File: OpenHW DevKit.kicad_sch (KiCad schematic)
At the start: 69 parts, among them J10 Conn_01x20, J4 Conn_01x02_Male, J7 Conn_01x20, J8 Conn_01x20, J9 Conn_01x20, Q1 MMBT3904, Q2 MMBT3904, SW1 SW_Push, SW2 SW_Push, U14 CORE-V-MCU, U3 W25Q32JWZP, U4 FXMA2102UMX, U6 NTB0104BQ,115, U7 NTB0104BQ,115, U8 NTB0104BQ,115, U9 NTB0104BQ,115, X1 ECS-2520MVLC-100-CN

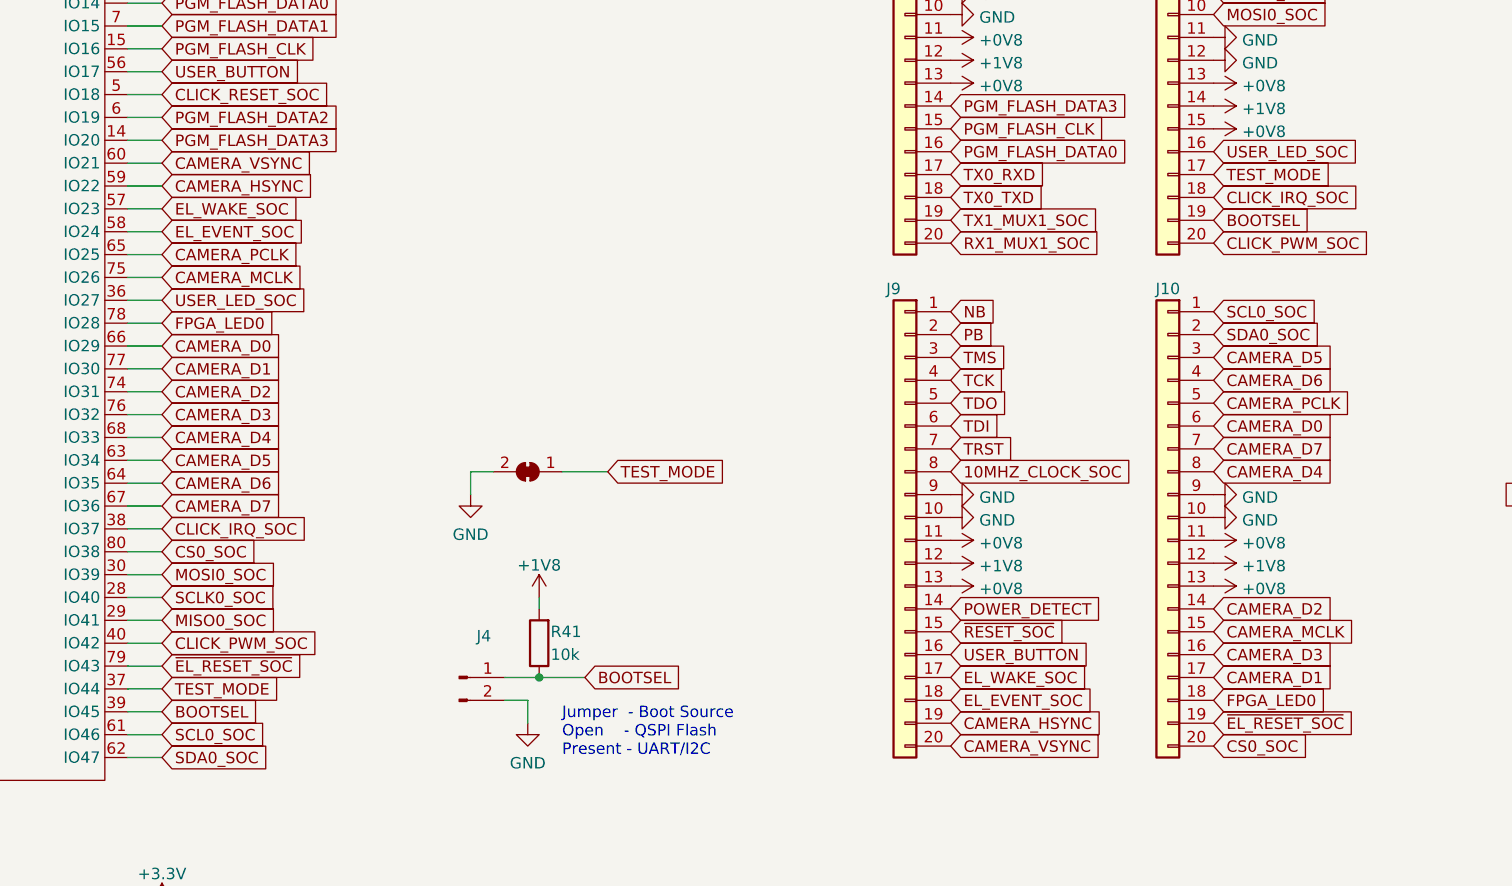
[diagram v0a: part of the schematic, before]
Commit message: swapped bootsel & test_mode pins
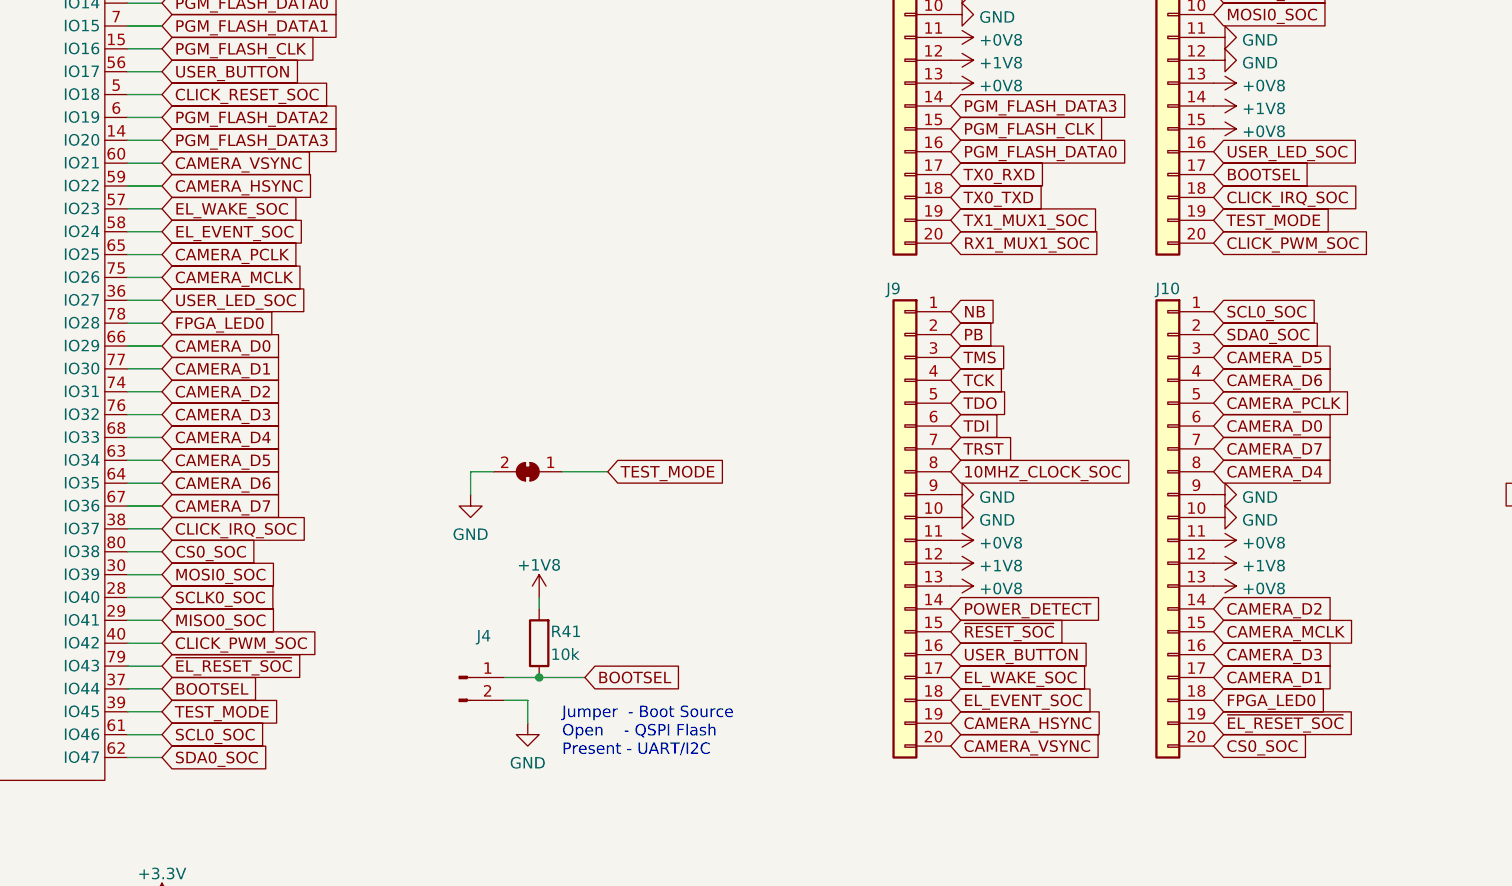
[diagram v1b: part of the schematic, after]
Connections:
- net BOOTSEL: now also J8.17 (Pin_17), U14.37 (IO44); no longer J8.19 (Pin_19), U14.39 (IO45)
- net TEST_MODE: now also J8.19 (Pin_19), U14.39 (IO45); no longer J8.17 (Pin_17), U14.37 (IO44)

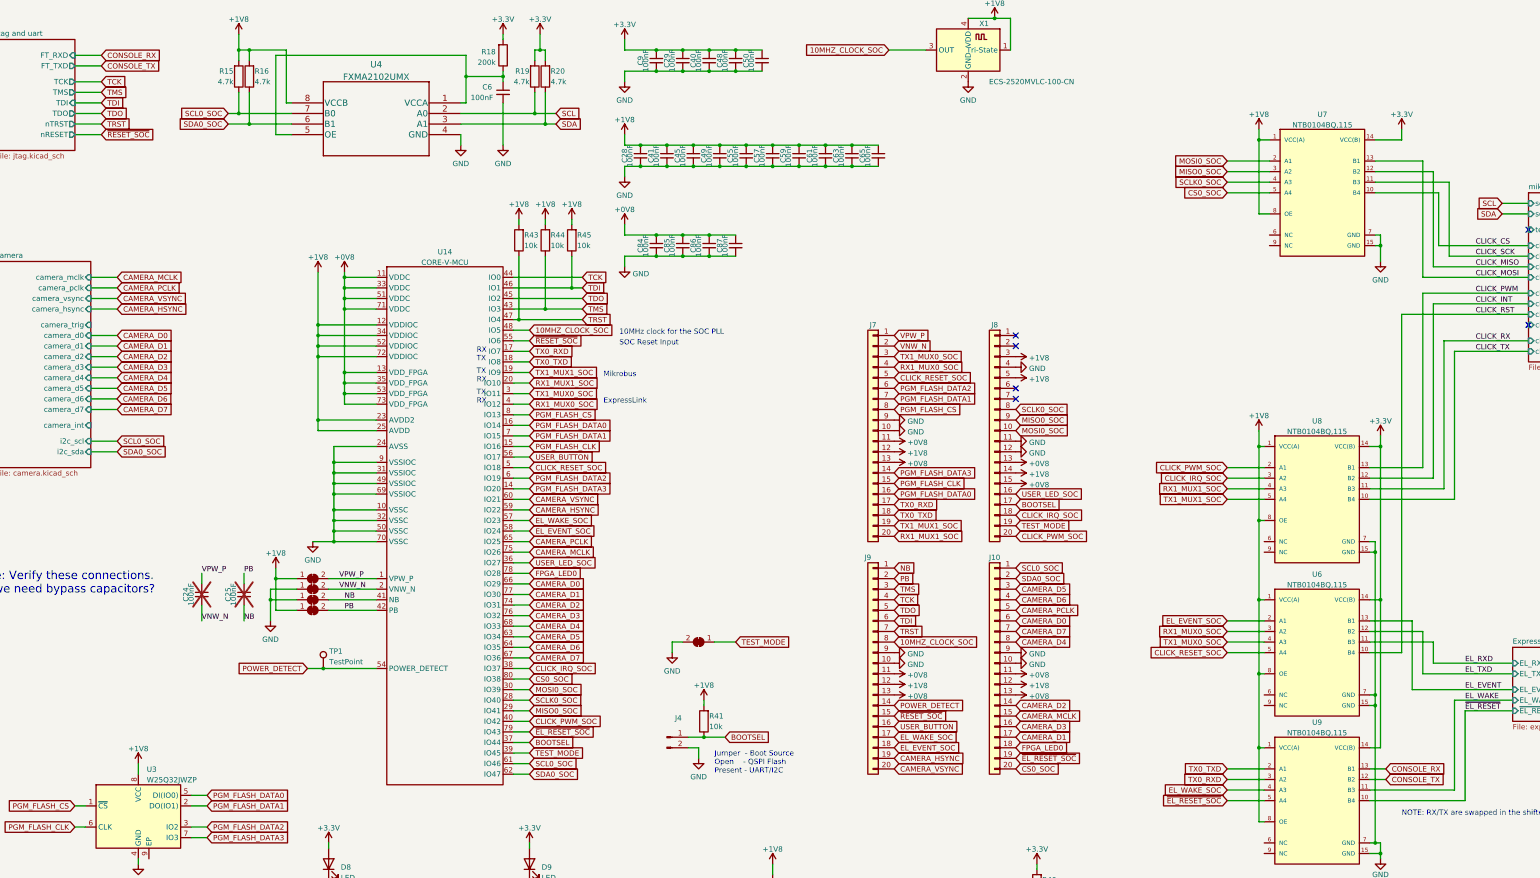
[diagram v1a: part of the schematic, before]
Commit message: updated footprints, added the barrel power connector and test points
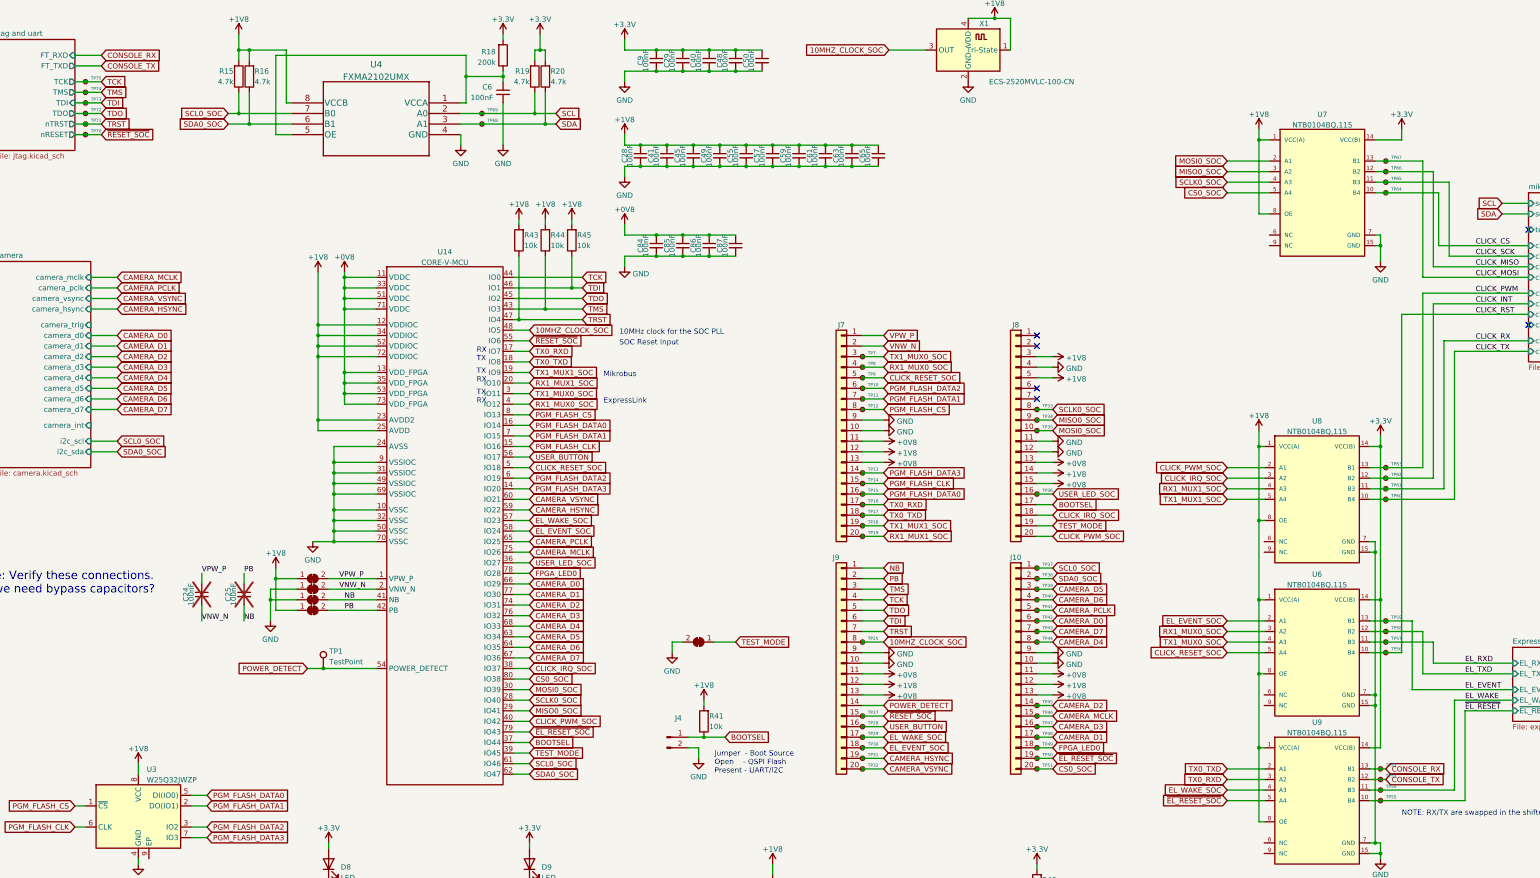
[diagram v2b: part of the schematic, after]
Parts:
- added TP10, TP11, TP12, TP13, TP14, TP15, TP16, TP17, TP18, TP19, TP25, TP27, TP28, TP29, TP30, TP31, TP32, TP33, TP34, TP35, TP36, TP37, TP38, TP39, TP40, TP41, TP42, TP43, TP44, TP45, TP46, TP47, TP48, TP49, TP50, TP51, TP52, TP53, TP54, TP55, TP56, TP57, TP58, TP59, TP60, TP61, TP62, TP63, TP64, TP65, TP66, TP67, TP68, TP69, TP7, TP70, TP71, TP72, TP73, TP74, TP75, TP8, TP9: TestPoint_Small, TestPoint:TestPoint_Pad_D1.0mm, symbol Connector:TestPoint_Small
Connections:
- net 10MHZ_CLOCK_SOC: now also TP25.1
- net CAMERA_D0: now also TP42.1
- net CAMERA_D1: now also TP48.1
- net CAMERA_D2: now also TP45.1
- net CAMERA_D3: now also TP47.1
- net CAMERA_D4: now also TP44.1
- net CAMERA_D5: now also TP39.1
- net CAMERA_D6: now also TP40.1
- net CAMERA_D7: now also TP43.1
- net CAMERA_HSYNC: now also TP31.1
- net CAMERA_MCLK: now also TP46.1
- net CAMERA_PCLK: now also TP41.1
- net CAMERA_VSYNC: now also TP32.1
- net CLICK_CS: now also TP64.1
- net CLICK_INT: now also TP62.1
- net CLICK_MISO: now also TP66.1
- net CLICK_MOSI: now also TP67.1
- net CLICK_PWM: now also TP63.1
- net CLICK_RESET_SOC: now also TP9.1
- net CLICK_RST: now also TP56.1
- net CLICK_RX: now also TP61.1
- net CLICK_SCK: now also TP65.1
- net CLICK_TX: now also TP60.1
- net CONSOLE_RX: now also TP52.1
- net CONSOLE_TX: now also TP53.1
- net CS0_SOC: now also TP51.1
- net EL_EVENT: now also TP59.1
- net EL_EVENT_SOC: now also TP30.1
- net EL_RXD: now also TP57.1
- net EL_TXD: now also TP58.1
- net EL_WAKE: now also TP54.1
- net EL_WAKE_SOC: now also TP29.1
- net FPGA_LED0: now also TP49.1
- net MISO0_SOC: now also TP34.1
- net MOSI0_SOC: now also TP35.1
- net PGM_FLASH_CLK: now also TP14.1
- net PGM_FLASH_CS: now also TP12.1
- net PGM_FLASH_DATA0: now also TP15.1
- net PGM_FLASH_DATA1: now also TP11.1
- net PGM_FLASH_DATA2: now also TP10.1
- net PGM_FLASH_DATA3: now also TP13.1
- net RX1_MUX0_SOC: now also TP8.1
- net RX1_MUX1_SOC: now also TP19.1
- net SCL: now also TP69.1
- net SCL0_SOC: now also TP37.1
- net SCLK0_SOC: now also TP33.1
- net SDA: now also TP68.1
- net SDA0_SOC: now also TP38.1
- net TCK: now also TP75.1
- net TDI: now also TP73.1
- net TDO: now also TP72.1
- net TMS: now also TP74.1
- net TRST: now also TP71.1
- net TX0_RXD: now also TP16.1
- net TX0_TXD: now also TP17.1
- net TX1_MUX0_SOC: now also TP7.1
- net TX1_MUX1_SOC: now also TP18.1
- net USER_BUTTON: now also TP28.1
- net USER_LED_SOC: now also TP36.1
- net ~{EL_RESET_SOC}: now also TP50.1
- net ~{EL_RESET}: now also TP55.1
- net ~{RESET_SOC}: now also TP27.1, TP70.1
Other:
- moved on the sheet: J10, J7, J8, J9
